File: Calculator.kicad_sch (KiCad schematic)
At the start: 24 parts, among them SW1 SW_Push, U1 ATmega32U4-A, Y1 16MHz

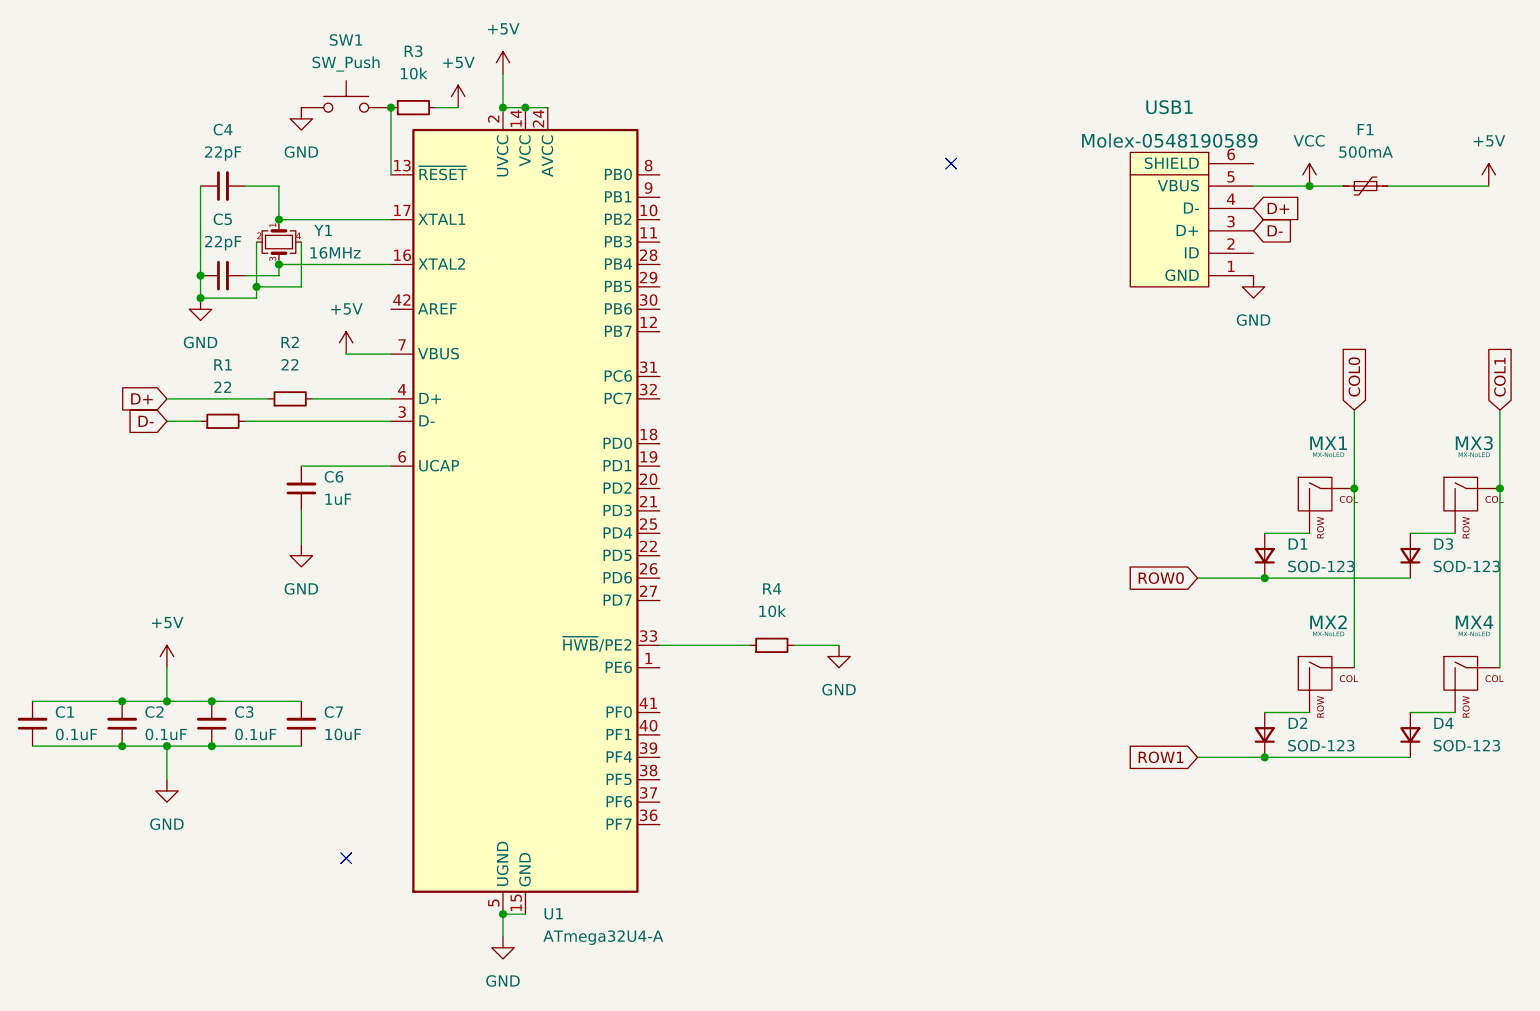
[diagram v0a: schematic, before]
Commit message: Add PCB
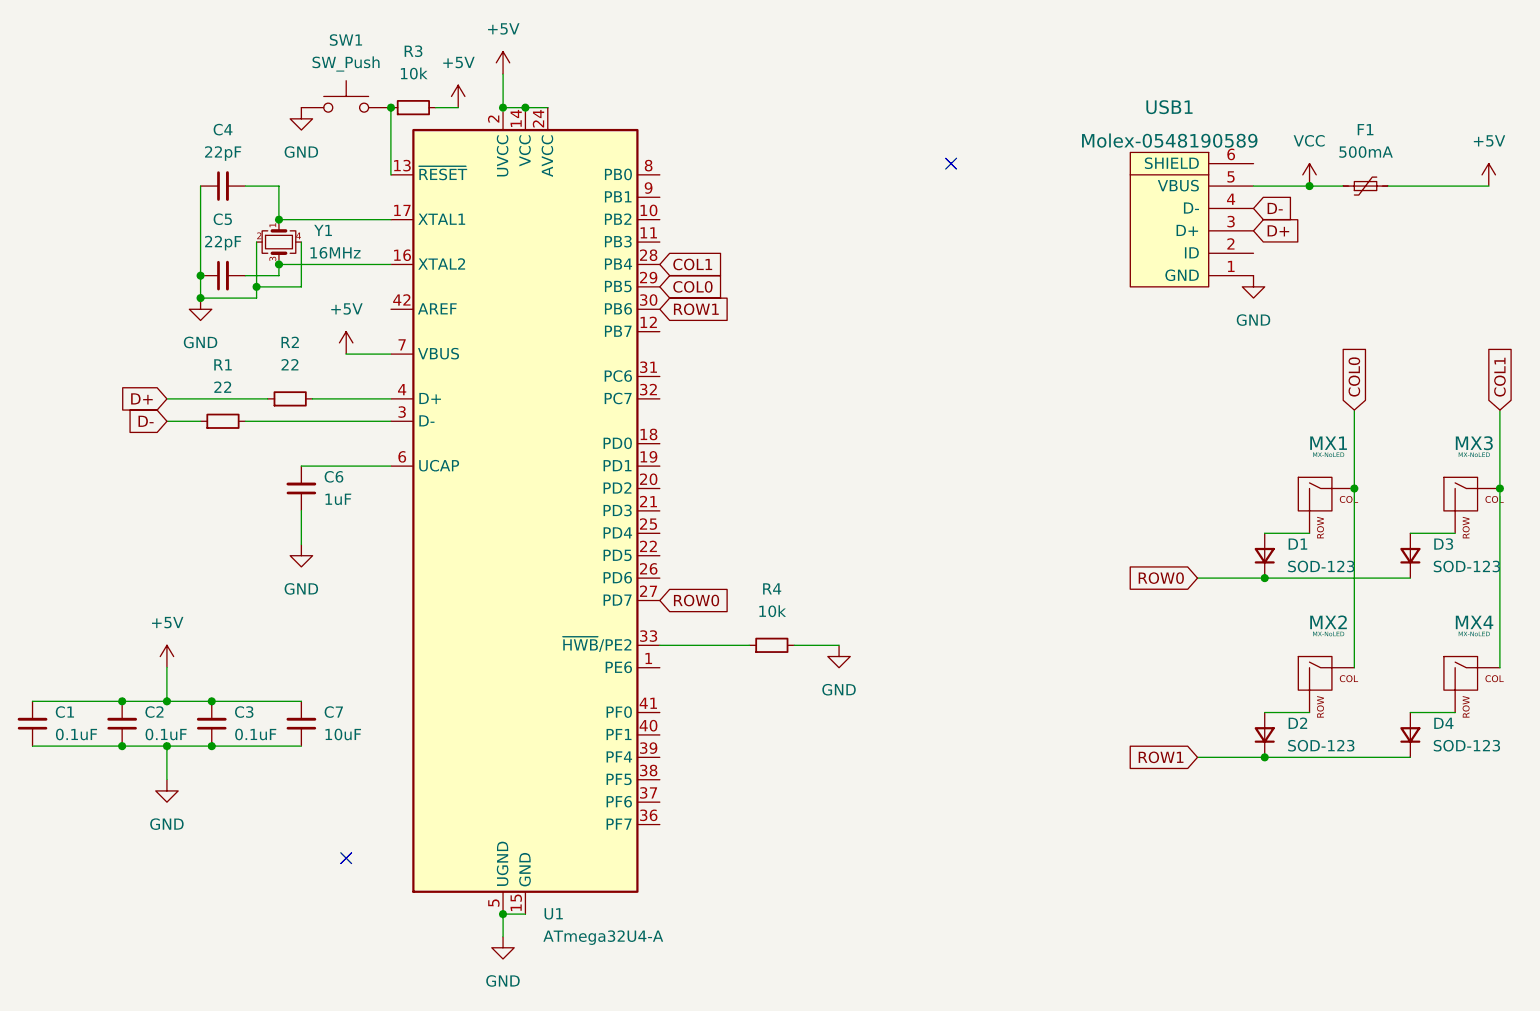
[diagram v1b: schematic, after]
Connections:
- net COL0: now also U1.29 (PB5)
- net COL1: now also U1.28 (PB4)
- net D+: now also USB1.3 (D+); no longer USB1.4 (D-)
- net D-: now also USB1.4 (D-); no longer USB1.3 (D+)
- net ROW0: now also U1.27 (PD7)
- net ROW1: now also U1.30 (PB6)
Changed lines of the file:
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@@
+    )
+  )
+  (global_label "ROW1" (shape input) (at 97.79 69.85 0) (fields_autoplaced)
+    (effects (font (size 1.27 1.27)) (justify left))
+    (property "Intersheet References" "${INTERSHEET_REFS}" (id 0) (at 105.4645 69.7706 0)
+      (effects (font (size 1.27 1.27)) (justify left) hide)
     )
   )
@@
     )
   )
-  (global_label "D+" (shape input) (at 165.1 58.42 0) (fields_autoplaced)
+  (global_label "COL0" (shape input) (at 97.79 67.31 0) (fields_autoplaced)
+    (effects (font (size 1.27 1.27)) (justify left))
+    (property "Intersheet References" "${INTERSHEET_REFS}" (id 0) (at 105.0412 67.2306 0)
+      (effects (font (size 1.27 1.27)) (justify left) hide)
+    )
+  )
+  (global_label "D-" (shape input) (at 165.1 58.42 0) (fields_autoplaced)
     (effects (font (size 1.27 1.27)) (justify left))
     (property "Intersheet References" "${INTERSHEET_REFS}" (id 0) (at 170.3555 58.3406 0)
@@
     )
   )
-  (global_label "D-" (shape input) (at 165.1 60.96 0) (fields_autoplaced)
+  (global_label "D+" (shape input) (at 165.1 60.96 0) (fields_autoplaced)
     (effects (font (size 1.27 1.27)) (justify left))
     (property "Intersheet References" "${INTERSHEET_REFS}" (id 0) (at 170.3555 60.8806 0)
       (effects (font (size 1.27 1.27)) (justify left) hide)
     )
+  )
+  (global_label "ROW0" (shape input) (at 97.79 102.87 0) (fields_autoplaced)
+    (effects (font (size 1.27 1.27)) (justify left))
+    (property "Intersheet References" "${INTERSHEET_REFS}" (id 0) (at 105.4645 102.7906 0)
+      (effects (font (size 1.27 1.27)) (justify left) hide)
+    )
+  )
+  (global_label "COL1" (shape input) (at 97.79 64.77 0) (fields_autoplaced)
+    (effects (font (size 1.27 1.27)) (justify left))
+    (property "Intersheet References" "${INTERSHEET_REFS}" (id 0) (at 105.0412 64.6906 0)
+      (effects (font (size 1.27 1.27)) (justify left) hide)
+    )
